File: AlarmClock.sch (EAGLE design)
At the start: 20 parts, among them IC1 LD1117AS33TR, T1 BC817-25LT1SMD

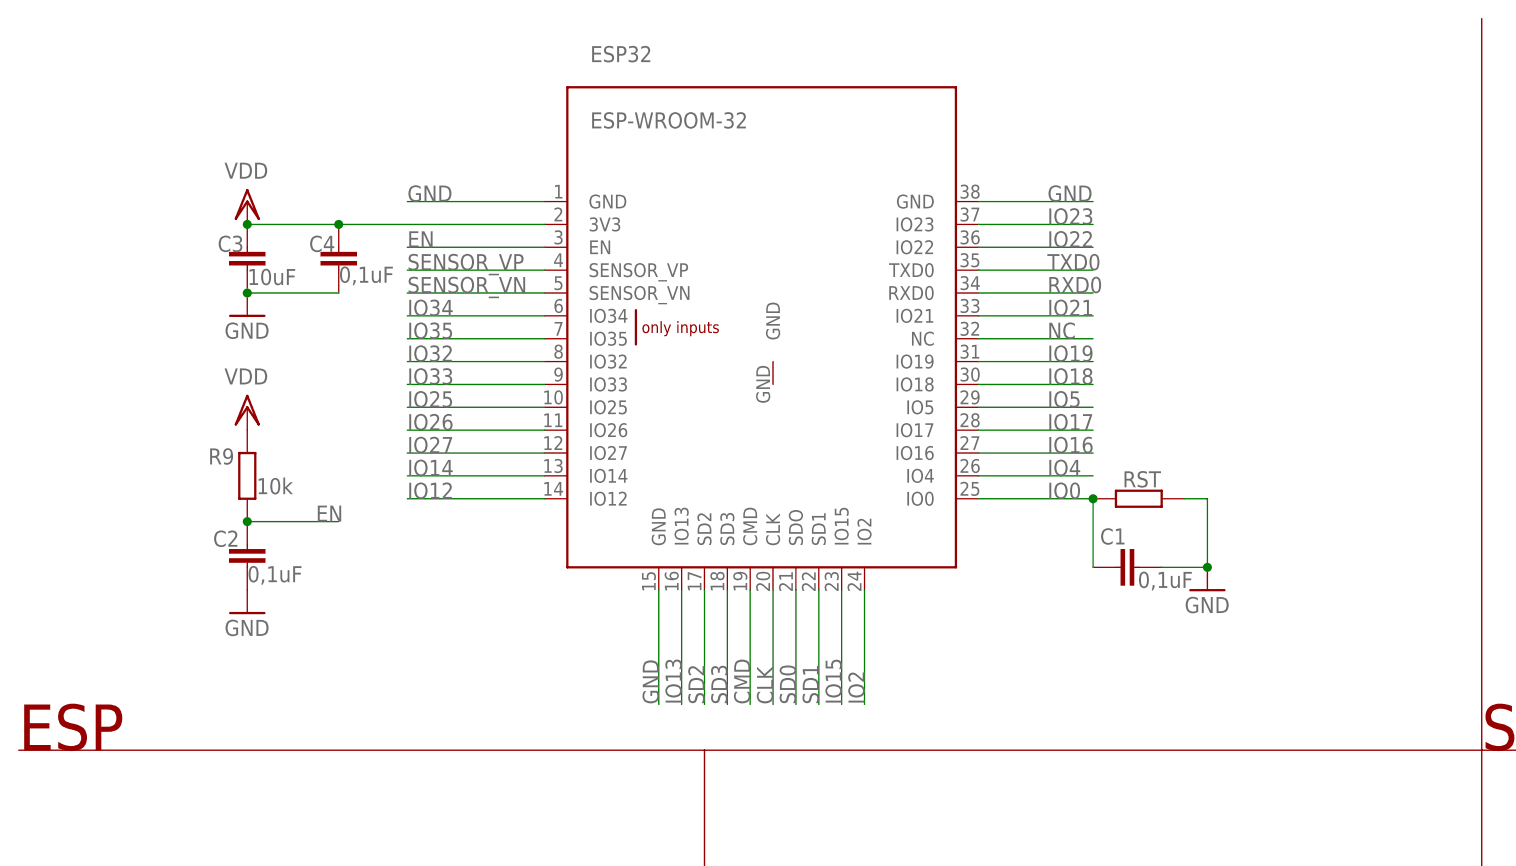
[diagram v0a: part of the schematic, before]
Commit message: Add files via upload
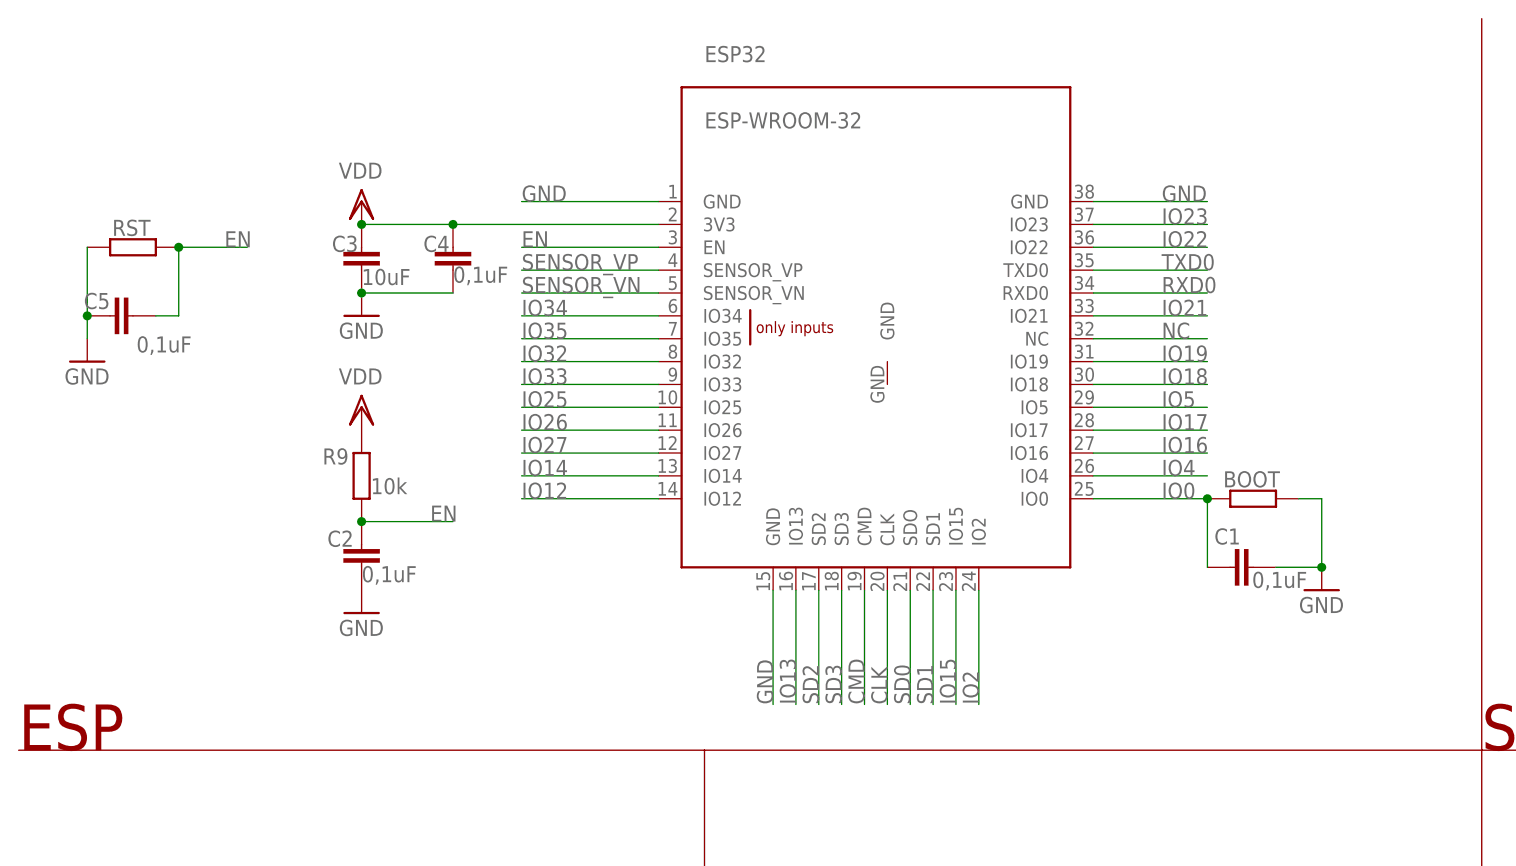
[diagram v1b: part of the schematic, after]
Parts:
- added BOOT: (no value), rcl:R-EU_R1206
- added C5: 0,1uF, rcl:C-EUC1206
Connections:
- net EN: now also C5.2, RST.2
- net GND: now also BOOT.2, C5.1, RST.1; no longer RST.2
- net IO0: now also BOOT.1; no longer RST.1
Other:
- moved on the sheet: C1, C2, C3, C4, ESP32, R9, RST
